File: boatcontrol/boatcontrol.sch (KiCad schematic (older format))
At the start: 343 parts, among them J1 TBL008V-1000-02BE, J10 TBL008V-1000-08BE, J11 TBL008V-1000-02BE, J12 TBL008V-1000-08BE, J2 SS73100-047F, J3 SS73100-047F, J4 TBP01R2W-508-08BE, J5 TBP01R2W-508-16BE, J6 TBP01R2W-508-08BE, J7 RPi_GPIO, J8 TBL008V-1000-02BE, J9 TBL008V-1000-02BE, K1 G5RL-K1A-E-DC12, K10 G5RL-K1A-E-DC12, K11 G5RL-K1A-E-DC12, K12 G5RL-K1A-E-DC12, K13 G5RL-K1A-E-DC12, K14 G5RL-K1A-E-DC12, K15 G5RL-K1A-E-DC12, K16 G5RL-K1A-E-DC12, K17 G5RL-K1A-E-DC12, K18 G5RL-K1A-E-DC12, K19 G5RL-K1A-E-DC12, K2 G5RL-K1A-E-DC12, K20 G5RL-K1A-E-DC12, K21 G5RL-K1A-E-DC12, K22 G5RL-K1A-E-DC12, K23 G5RL-K1A-E-DC12, K24 G5RL-K1A-E-DC12, K25 G5RL-K1A-E-DC12, K26 G5RL-K1A-E-DC12, K27 G5RL-K1A-E-DC12, K28 G5RL-K1A-E-DC12, K29 G5RL-K1A-E-DC12, K3 G5RL-K1A-E-DC12, K30 G5RL-K1A-E-DC12, K31 G5RL-K1A-E-DC12, K32 G5RL-K1A-E-DC12, K33 EW60-1A3-CL12D04, K34 EW60-1A3-CL12D04, K35 EW60-1A3-CL12D04, K36 EW60-1A3-CL12D04, K37 EW60-1A3-CL12D04, K38 EW60-1A3-CL12D04, K39 EW60-1A3-CL12D04, K4 G5RL-K1A-E-DC12, K40 EW60-1A3-CL12D04, K5 G5RL-K1A-E-DC12, K6 G5RL-K1A-E-DC12, K7 G5RL-K1A-E-DC12, K8 G5RL-K1A-E-DC12, K9 G5RL-K1A-E-DC12, Q1 SchurterCircuitBreaker 3a, Q10 SchurterCircuitBreaker 3a, Q11 SchurterCircuitBreaker 3a, Q12 SchurterCircuitBreaker 3a, Q13 SchurterCircuitBreaker 3a, Q14 SchurterCircuitBreaker 3a, Q15 SchurterCircuitBreaker 3a, Q16 SchurterCircuitBreaker 3a, Q17 SchurterCircuitBreaker 6a, Q18 SchurterCircuitBreaker 6a, Q19 SchurterCircuitBreaker 6a, Q2 SchurterCircuitBreaker 3a, Q20 SchurterCircuitBreaker 6a, Q21 SchurterCircuitBreaker 10a, Q22 SchurterCircuitBreaker 10a, Q23 SchurterCircuitBreaker 16a, Q24 SchurterCircuitBreaker 16a, Q25 SchurterCircuitBreaker 6a, Q26 SchurterCircuitBreaker 6a, Q27 SchurterCircuitBreaker 6a, Q28 SchurterCircuitBreaker 6a, Q29 SchurterCircuitBreaker 10a, Q3 SchurterCircuitBreaker 3a, Q30 SchurterCircuitBreaker 10a, Q31 SchurterCircuitBreaker 16a, Q32 SchurterCircuitBreaker 16a, Q33 SchurterCircuitBreaker 3a, Q4 SchurterCircuitBreaker 3a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

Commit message: Split 60A to own daughter board.
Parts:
- removed J7: RPi_GPIO, BoatControl:Samtec_HLE-120-02-XXX-DV-BE-XX-XX, symbol boatcontrol-rescue:RPi_GPIO-RPi_Hat-rescue
- added J?: Raspberry_Pi_2_3, Connector_PinSocket_2.00mm:PinSocket_2x20_P2.00mm_Vertical, symbol Connector:Raspberry_Pi_2_3
- added J?: Conn_02x20_Odd_Even Header, Connector_PinSocket_2.00mm:PinSocket_2x20_P2.00mm_Vertical, symbol Connector_Generic:Conn_02x20_Odd_Even
- added J?: Conn_02x20_Odd_Even Socket, Connector_PinHeader_2.00mm:PinHeader_2x20_P2.00mm_Vertical, symbol Connector_Generic:Conn_02x20_Odd_Even
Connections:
- net D33A: no longer D33.1 (A1), RN2.9 (R8.2)
- net D33B: no longer D33.3 (A2), RN1.9 (R8.2), RN2.10 (R7.2)
- net D34A: no longer D34.1 (A1), RN2.11 (R6.2)
- net D34B: no longer D34.3 (A2), RN2.12 (R5.2)
- net D35A: no longer D35.1 (A1), RN2.13 (R4.2)
- net D35B: no longer D35.3 (A2), RN2.14 (R3.2)
- net D36A: no longer D36.1 (A1), RN2.15 (R2.2)
- net D36B: no longer D36.3 (A2), RN2.16 (R1.2)
- net D37A: no longer D37.1 (A1), RN1.16 (R1.2)
- net D37B: no longer D37.3 (A2), RN1.15 (R2.2)
- net D38A: no longer D38.1 (A1), RN1.14 (R3.2)
- net D38B: no longer D38.3 (A2), RN1.13 (R4.2)
- net D39A: no longer D39.1 (A1), RN1.12 (R5.2)
- net D39B: no longer D39.3 (A2), RN1.11 (R6.2)
- net D40A: no longer D40.1 (A1), RN1.10 (R7.2)
- net K33A: now also J?.1 (Pin_1); no longer RN2.8 (R8.1), SW33A1.2 (B), SW33A1.5 (B)
- net K33B: now also J?.2 (Pin_2); no longer RN1.8 (R8.1), RN2.7 (R7.1), SWSW33B1.2 (B), SWSW33B1.5 (B)
- net K34A: now also J?.3 (Pin_3); no longer RN2.6 (R6.1), SW34A1.2 (B), SW34A1.5 (B)
- net K34B: now also J?.4 (Pin_4); no longer RN2.5 (R5.1)
- net K35A: now also J?.5 (Pin_5); no longer RN2.4 (R4.1), SW35A1.2 (B), SW35A1.5 (B)
- net K35B: now also J?.6 (Pin_6); no longer RN2.3 (R3.1)
- net K36A: now also J?.7 (Pin_7); no longer RN2.2 (R2.1), SW36A1.2 (B), SW36A1.5 (B)
- net K36B: now also J?.8 (Pin_8); no longer RN2.1 (R1.1)
- net K37A: no longer RN1.1 (R1.1), SW37A1.2 (B), SW37A1.5 (B)
- net K37B: no longer RN1.2 (R2.1)
- net K38A: now also J?.9 (Pin_9); no longer RN1.3 (R3.1), SW38A1.2 (B), SW38A1.5 (B)
- net K38B: now also J?.10 (Pin_10); no longer RN1.4 (R4.1), SW38B1.2 (B), SW38B1.5 (B)
- net K39A: now also J?.11 (Pin_11); no longer RN1.5 (R5.1), SW39A1.2 (B), SW39A1.5 (B)
- net K39B: now also J?.12 (Pin_12); no longer RN1.6 (R6.1), SW39B1.2 (B), SW39B1.5 (B)
- net K40A: now also K40.A3, J?.13 (Pin_13); no longer RN1.7 (R7.1)
- net K40B: now also J?.14 (Pin_14)
- net at K33.1, K33.2, K33.3: now also J10.1_1 (01P), J10.1_2 (01P), J10.1_3 (01P); no longer J12.1_1 (01P), J12.1_2 (01P), J12.1_3 (01P)
- net at K33.4, K33.5, K33.6: now also J12.1_1 (01P), J12.1_2 (01P), J12.1_3 (01P); no longer J10.1_1 (01P), J10.1_2 (01P), J10.1_3 (01P)
- net at K33.A1, K34.A1, K35.A1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: now also J?.27 (Pin_27), J?.28 (Pin_28), J?.29 (Pin_29), J?.30 (Pin_30), J?.31 (Pin_31), J?.32 (Pin_32), J?.33 (Pin_33), J?.34 (Pin_34), J?.35 (Pin_35), J?.36 (Pin_36), J?.37 (Pin_37), J?.38 (Pin_38), J?.39 (Pin_39), J?.40 (Pin_40); no longer D33.2 (K), D34.2 (K), D35.2 (K), D36.2 (K), D37.2 (K), D38.2 (K), D39.2 (K), D40.2 (K)
- net at K34.1, K34.2, K34.3: now also J10.2_1 (02P), J10.2_2 (02P), J10.2_3 (02P); no longer J12.2_1 (02P), J12.2_2 (02P), J12.2_3 (02P)
- net at K34.4, K34.5, K34.6: now also J12.2_1 (02P), J12.2_2 (02P), J12.2_3 (02P); no longer J10.2_1 (02P), J10.2_2 (02P), J10.2_3 (02P)
- net at K35.1, K35.2, K35.3: now also J10.3_1 (03P), J10.3_2 (03P), J10.3_3 (03P); no longer J12.3_1 (03P), J12.3_2 (03P), J12.3_3 (03P)
- net at K35.4, K35.5, K35.6: now also J12.3_1 (03P), J12.3_2 (03P), J12.3_3 (03P); no longer J10.3_1 (03P), J10.3_2 (03P), J10.3_3 (03P)
- net at K36.1, K36.2, K36.3: now also J10.4_1 (04P), J10.4_2 (04P), J10.4_3 (04P); no longer J12.4_1 (04P), J12.4_2 (04P), J12.4_3 (04P)
- net at K36.4, K36.5, K36.6: now also J12.4_1 (04P), J12.4_2 (04P), J12.4_3 (04P); no longer J10.4_1 (04P), J10.4_2 (04P), J10.4_3 (04P)
- net at K37.1, K37.2, K37.3: now also J10.5_1 (05P), J10.5_2 (05P), J10.5_3 (05P); no longer J12.5_1 (05P), J12.5_2 (05P), J12.5_3 (05P)
- net at K37.4, K37.5, K37.6: now also J12.5_1 (05P), J12.5_2 (05P), J12.5_3 (05P); no longer J10.5_1 (05P), J10.5_2 (05P), J10.5_3 (05P)
- net at K38.1, K38.2, K38.3: now also J10.6_1 (06P), J10.6_2 (06P), J10.6_3 (06P); no longer J12.6_1 (06P), J12.6_2 (06P), J12.6_3 (06P)
- net at K38.4, K38.5, K38.6: now also J12.6_1 (06P), J12.6_2 (06P), J12.6_3 (06P); no longer J10.6_1 (06P), J10.6_2 (06P), J10.6_3 (06P)
- net at K39.1, K39.2, K39.3: now also J10.7_1 (07P), J10.7_2 (07P), J10.7_3 (07P); no longer J12.7_1 (07P), J12.7_2 (07P), J12.7_3 (07P)
- net at K39.4, K39.5, K39.6: now also J12.7_1 (07P), J12.7_2 (07P), J12.7_3 (07P); no longer J10.7_1 (07P), J10.7_2 (07P), J10.7_3 (07P)
- net at K40.1, K40.2, K40.3: now also J10.8_1 (08P), J10.8_2 (08P), J10.8_3 (08P); no longer J12.8_1 (08P), J12.8_2 (08P), J12.8_3 (08P)
- net at K40.4, K40.5, K40.6: now also J12.8_1 (08P), J12.8_2 (08P), J12.8_3 (08P); no longer J10.8_1 (08P), J10.8_2 (08P), J10.8_3 (08P)
- net at U19.21 (GPA0): no longer U21.11 (O8)
- net at U19.22 (GPA1): no longer U21.12 (O7)
- net at U19.23 (GPA2): no longer U21.13 (O6)
- net at U19.24 (GPA3): no longer U21.14 (O5)
- net at U19.5 (GPB4): no longer U20.15 (O4)
- net at U19.6 (GPB5): no longer U20.16 (O3)
- net at U19.7 (GPB6): no longer U20.17 (O2)
- net at U19.8 (GPB7): no longer U20.18 (O1)
- net at SW40B1.2 (B): no longer SW40B1.5 (B)
- net D40B: no longer names the net of D40.3 (A2)
- new net: D33.1 (A1), RN2.1 (R1.1)
- new net: D33.3 (A2), RN1.1 (R1.1)
- new net: D34.1 (A1), RN2.2 (R2.1)
- new net: D34.3 (A2), RN1.2 (R2.1)
- new net: D35.1 (A1), RN2.3 (R3.1)
- new net: D35.3 (A2), RN1.3 (R3.1)
- new net: D36.1 (A1), RN2.4 (R4.1)
- new net: D36.3 (A2), RN1.4 (R4.1)
- new net: D37.1 (A1), RN2.5 (R5.1)
- new net: D37.3 (A2), RN1.5 (R5.1)
- new net: D38.1 (A1), RN2.6 (R6.1)
- new net: D38.3 (A2), RN1.6 (R6.1)
- new net: D39.1 (A1), RN2.7 (R7.1)
- new net: D39.3 (A2), RN1.7 (R7.1)
- now unconnected: SW33A1.1 (A), SW33A1.3 (C), SW33A1.4 (A), SW33A1.6 (C), SW34A1.1 (A), SW34A1.3 (C), SW34A1.4 (A), SW34A1.6 (C), SW34B1.1 (A), SW34B1.3 (C), SW34B1.4 (A), SW34B1.6 (C), SW35A1.1 (A), SW35A1.3 (C), SW35A1.4 (A), SW35A1.6 (C), SW35B1.1 (A), SW35B1.3 (C), SW35B1.4 (A), SW35B1.6 (C), SW36A1.1 (A), SW36A1.3 (C), SW36A1.4 (A), SW36A1.6 (C), SW36B1.1 (A), SW36B1.3 (C), SW36B1.4 (A), SW36B1.6 (C), SW37A1.1 (A), SW37A1.3 (C), SW37A1.4 (A), SW37A1.6 (C), SW37B1.1 (A), SW37B1.3 (C), SW37B1.4 (A), SW37B1.6 (C), SW38A1.1 (A), SW38A1.3 (C), SW38A1.4 (A), SW38A1.6 (C), SW38B1.1 (A), SW38B1.3 (C), SW38B1.4 (A), SW38B1.6 (C), SW39A1.1 (A), SW39A1.3 (C), SW39A1.4 (A), SW39A1.6 (C), SW39B1.1 (A), SW39B1.3 (C), SW39B1.4 (A), SW39B1.6 (C), SW40A1.1 (A), SW40A1.2 (B), SW40A1.3 (C), SW40A1.4 (A), SW40A1.5 (B), SW40A1.6 (C), SW40B1.1 (A), SW40B1.3 (C), SW40B1.4 (A), SW40B1.6 (C), SWSW33B1.1 (A), SWSW33B1.3 (C), SWSW33B1.4 (A), SWSW33B1.6 (C), U20.1 (I1), U20.2 (I2), U20.3 (I3), U20.4 (I4), U20.5 (I5), U20.6 (I6), U20.7 (I7), U20.8 (I8), U21.1 (I1), U21.2 (I2), U21.3 (I3), U21.4 (I4), U21.5 (I5), U21.6 (I6), U21.7 (I7), U21.8 (I8), U21.9 (GND)
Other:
- moved on the sheet: D33, D34, D35, D36, D37, D38, D39, D40, J10, J12, K33, K34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

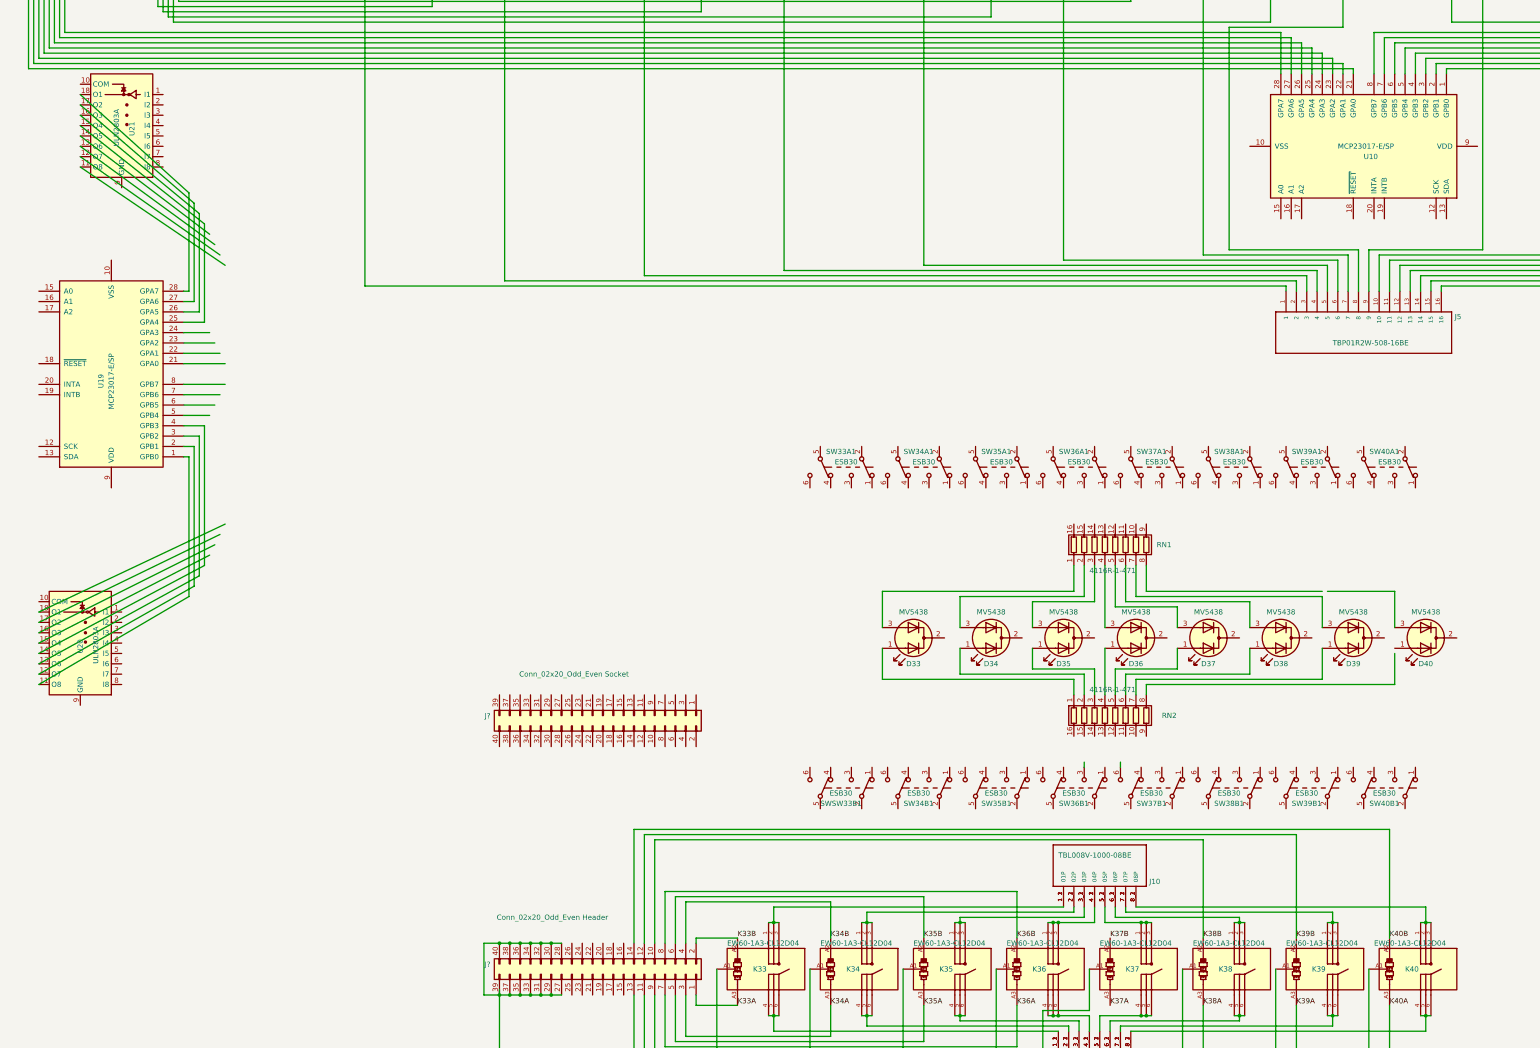
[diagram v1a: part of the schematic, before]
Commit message: Split high power
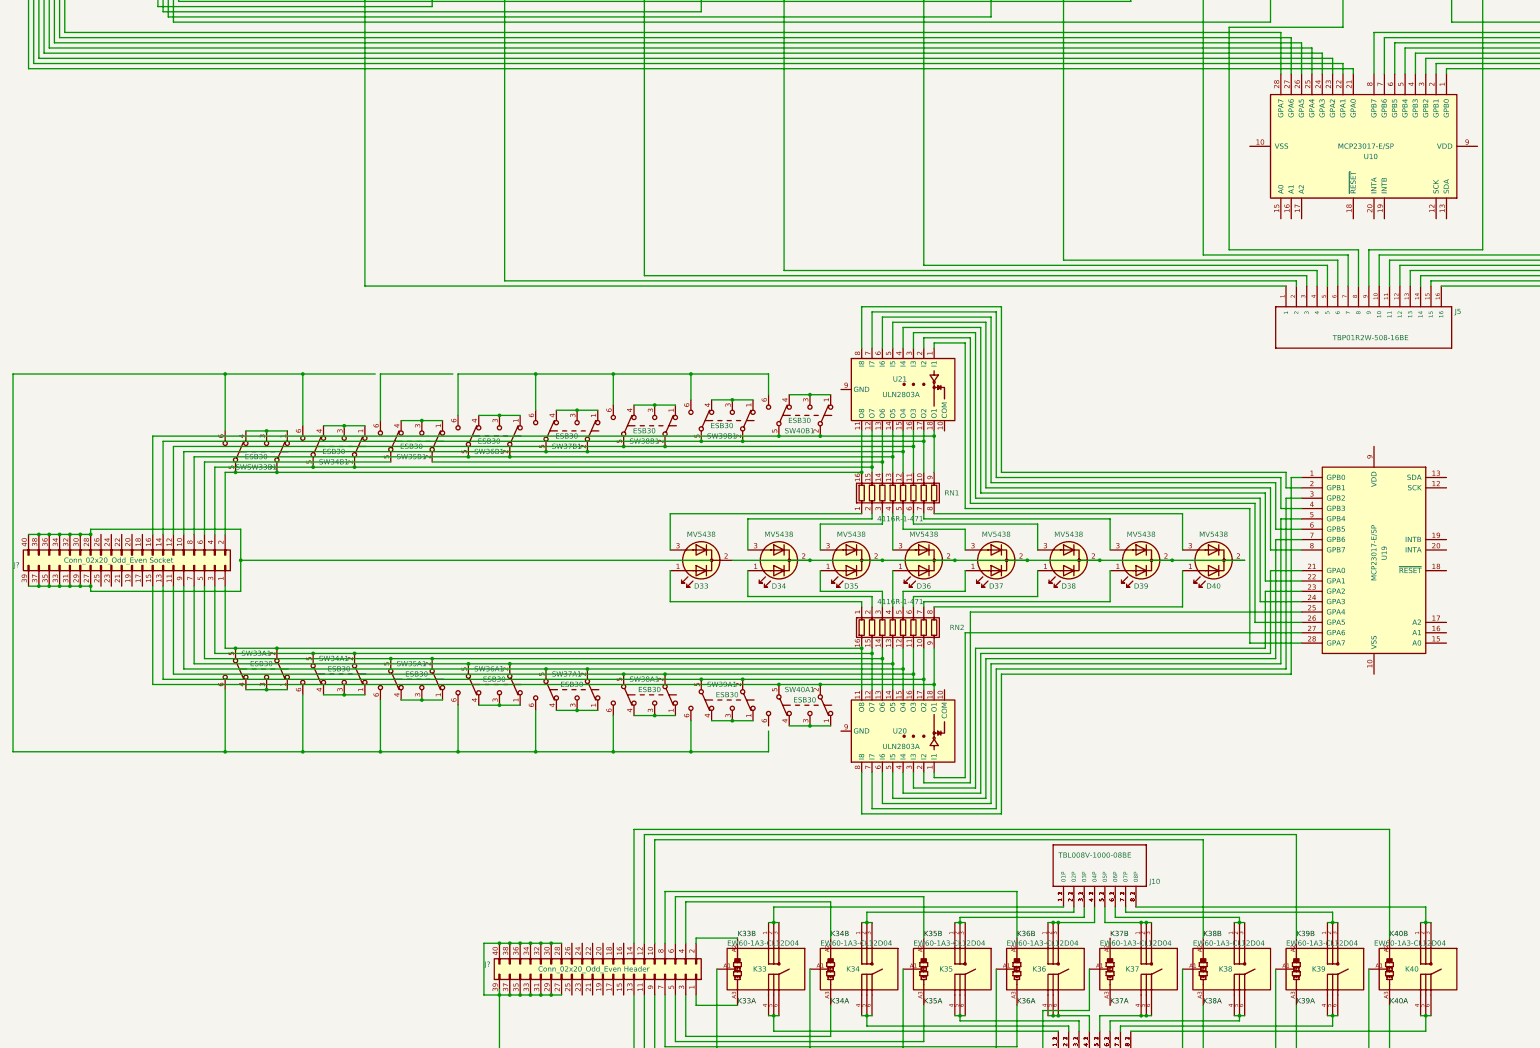
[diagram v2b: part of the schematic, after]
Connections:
- net at U19.1 (GPB0): now also U20.8 (I8); no longer U20.11 (O8)
- net at U19.2 (GPB1): now also U21.8 (I8); no longer U20.12 (O7)
- net at U19.21 (GPA0): now also U20.4 (I4)
- net at U19.22 (GPA1): now also U21.4 (I4)
- net at U19.23 (GPA2): now also U20.3 (I3)
- net at U19.24 (GPA3): now also U21.3 (I3)
- net at U19.25 (GPA4): now also U20.2 (I2); no longer U21.15 (O4)
- net at U19.26 (GPA5): now also U21.2 (I2); no longer U21.16 (O3)
- net at U19.27 (GPA6): now also U20.1 (I1); no longer U21.17 (O2)
- net at U19.28 (GPA7): now also U21.1 (I1); no longer U21.18 (O1)
- net at U19.3 (GPB2): now also U20.7 (I7); no longer U20.13 (O6)
- net at U19.4 (GPB3): now also U21.7 (I7); no longer U20.14 (O5)
- net at U19.5 (GPB4): now also U20.6 (I6)
- net at U19.6 (GPB5): now also U21.6 (I6)
- net at U19.7 (GPB6): now also U20.5 (I5)
- net at U19.8 (GPB7): now also U21.5 (I5)
- net at U20.15 (O4): now also J?.9 (Pin_9), RN2.12 (R5.2), SW37A1.2 (B), SW37A1.5 (B)
- net at U20.16 (O3): now also J?.11 (Pin_11), RN2.11 (R6.2), SW38A1.2 (B), SW38A1.5 (B)
- net at U20.17 (O2): now also J?.13 (Pin_13), RN2.10 (R7.2), SW39A1.2 (B), SW39A1.5 (B)
- net at U20.18 (O1): now also J?.15 (Pin_15), RN2.9 (R8.2), SW40A1.2 (B), SW40A1.5 (B)
- net at U21.11 (O8): now also J?.2 (Pin_2), RN1.16 (R1.2), SWSW33B1.2 (B), SWSW33B1.5 (B)
- net at U21.12 (O7): now also J?.4 (Pin_4), RN1.15 (R2.2), SW34B1.2 (B), SW34B1.5 (B)
- net at U21.13 (O6): now also RN1.14 (R3.2), SW35B1.2 (B)
- net at U21.14 (O5): now also J?.8 (Pin_8), RN1.13 (R4.2), SW36B1.2 (B), SW36B1.5 (B)
- net at D33.2 (K): now also D34.2 (K), D35.2 (K), D36.2 (K), D37.2 (K), D38.2 (K), D39.2 (K), D40.2 (K)
- net at D40.1 (A1): now also RN2.8 (R8.1)
- net at D40.3 (A2): now also RN1.8 (R8.1)
- net at RN2.13 (R4.2): now also J?.7 (Pin_7), SW36A1.2 (B), SW36A1.5 (B), U20.14 (O5)
- net at RN2.14 (R3.2): now also J?.5 (Pin_5), SW35A1.2 (B), SW35A1.5 (B), U20.13 (O6)
- net at RN2.15 (R2.2): now also J?.3 (Pin_3), SW34A1.2 (B), SW34A1.5 (B), U20.12 (O7)
- net at RN2.16 (R1.2): now also J?.1 (Pin_1), SW33A1.2 (B), SW33A1.5 (B), U20.11 (O8)
- net at RN1.10 (R7.2): now also J?.14 (Pin_14), SW39B1.2 (B), SW39B1.5 (B), U21.17 (O2)
- net at RN1.11 (R6.2): now also J?.12 (Pin_12), SW38B1.2 (B), SW38B1.5 (B), U21.16 (O3)
- net at RN1.12 (R5.2): now also J?.10 (Pin_10), SW37B1.2 (B), SW37B1.5 (B), U21.15 (O4)
- net at RN1.9 (R8.2): now also J?.16 (Pin_16), SW40B1.2 (B), SW40B1.5 (B), U21.18 (O1)
- net at J?.27 (Pin_27): now also J?.28 (Pin_28), J?.29 (Pin_29), J?.30 (Pin_30), J?.31 (Pin_31), J?.32 (Pin_32), J?.33 (Pin_33), J?.34 (Pin_34), J?.35 (Pin_35), J?.36 (Pin_36), J?.37 (Pin_37), J?.38 (Pin_38), J?.39 (Pin_39), J?.40 (Pin_40)
- net at J?.6 (Pin_6): now also SW35B1.5 (B)
- net at SWSW33B1.1 (A): now also SWSW33B1.3 (C), SWSW33B1.4 (A)
- net at SWSW33B1.6 (C): now also SW33A1.6 (C), SW34A1.6 (C), SW34B1.6 (C), SW35A1.6 (C), SW36A1.6 (C), SW37A1.6 (C), SW38A1.6 (C), SW39A1.6 (C)
- net at SW33A1.1 (A): now also SW33A1.3 (C), SW33A1.4 (A)
- net at SW34A1.1 (A): now also SW34A1.3 (C), SW34A1.4 (A)
- net at SW35A1.1 (A): now also SW35A1.3 (C), SW35A1.4 (A)
- net at SW36A1.1 (A): now also SW36A1.3 (C), SW36A1.4 (A)
- net at SW37A1.1 (A): now also SW37A1.3 (C), SW37A1.4 (A)
- net at SW38A1.1 (A): now also SW38A1.3 (C), SW38A1.4 (A)
- net at SW39A1.1 (A): now also SW39A1.3 (C), SW39A1.4 (A)
- net at SW40A1.1 (A): now also SW40A1.3 (C), SW40A1.4 (A)
- net at SW34B1.1 (A): now also SW34B1.3 (C), SW34B1.4 (A)
- net at SW35B1.1 (A): now also SW35B1.3 (C), SW35B1.4 (A)
- net at SW36B1.1 (A): now also SW36B1.3 (C), SW36B1.4 (A)
- net at SW36B1.6 (C): now also SW37B1.6 (C), SW38B1.6 (C), SW39B1.6 (C), SW40B1.6 (C)
- net at SW37B1.1 (A): now also SW37B1.3 (C), SW37B1.4 (A)
- net at SW38B1.1 (A): now also SW38B1.3 (C), SW38B1.4 (A)
- net at SW39B1.1 (A): now also SW39B1.3 (C), SW39B1.4 (A)
- net at SW40B1.1 (A): now also SW40B1.3 (C), SW40B1.4 (A)
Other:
- moved on the sheet: D33, D34, D35, D36, D37, D38, D39, D40, J5, J?, RN1, RN2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
